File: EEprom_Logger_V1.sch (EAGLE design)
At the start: 25 parts, among them IC1 AP2138N-3.3TRG1, IC2 PIC18F13K22SOP, IC3 MIC94090, IC4 MCP1700T-2702E/TT, IC5 24LC16BSN, Q1 Si2333CDS-T1-GE3, Q2 Si2333CDS-T1-GE3, Y1 32kHz

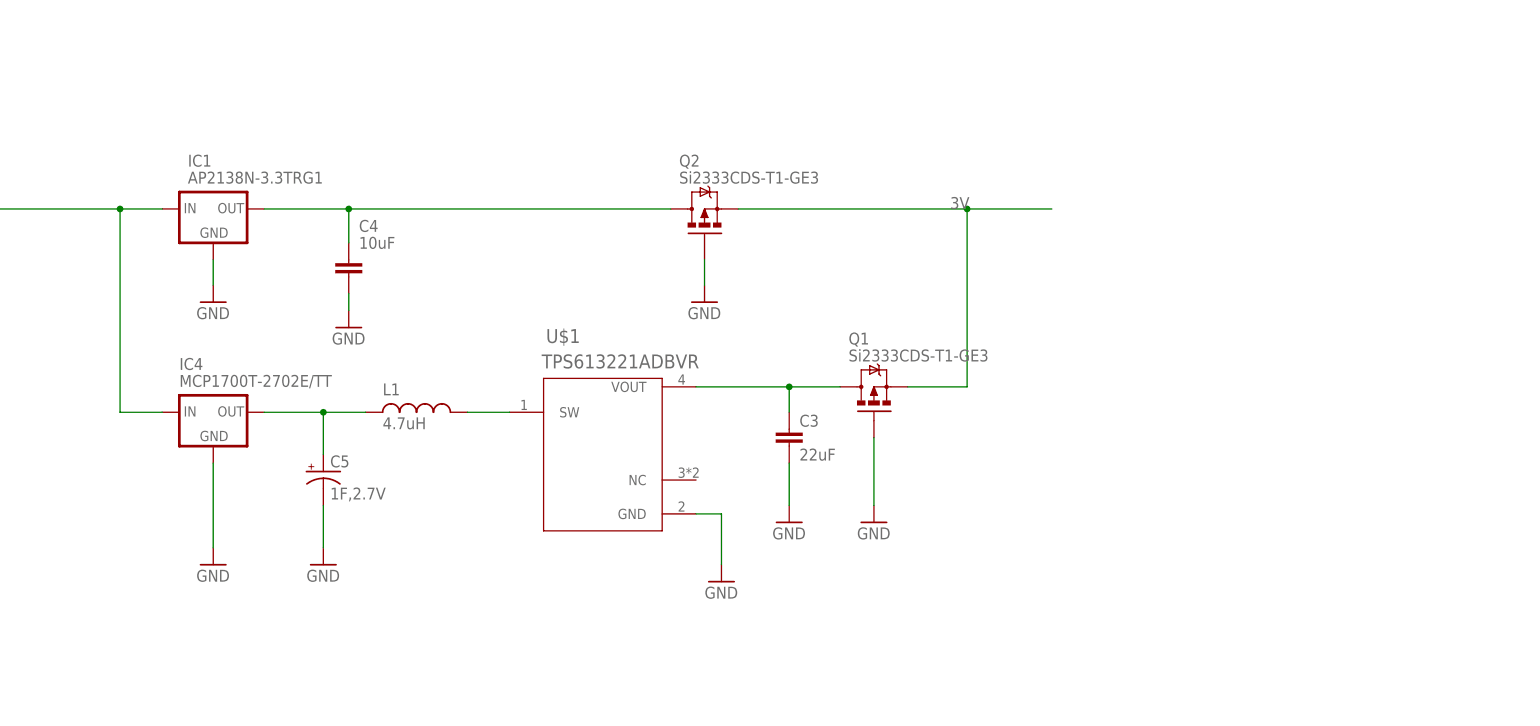
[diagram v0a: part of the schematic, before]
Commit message: Add files via upload
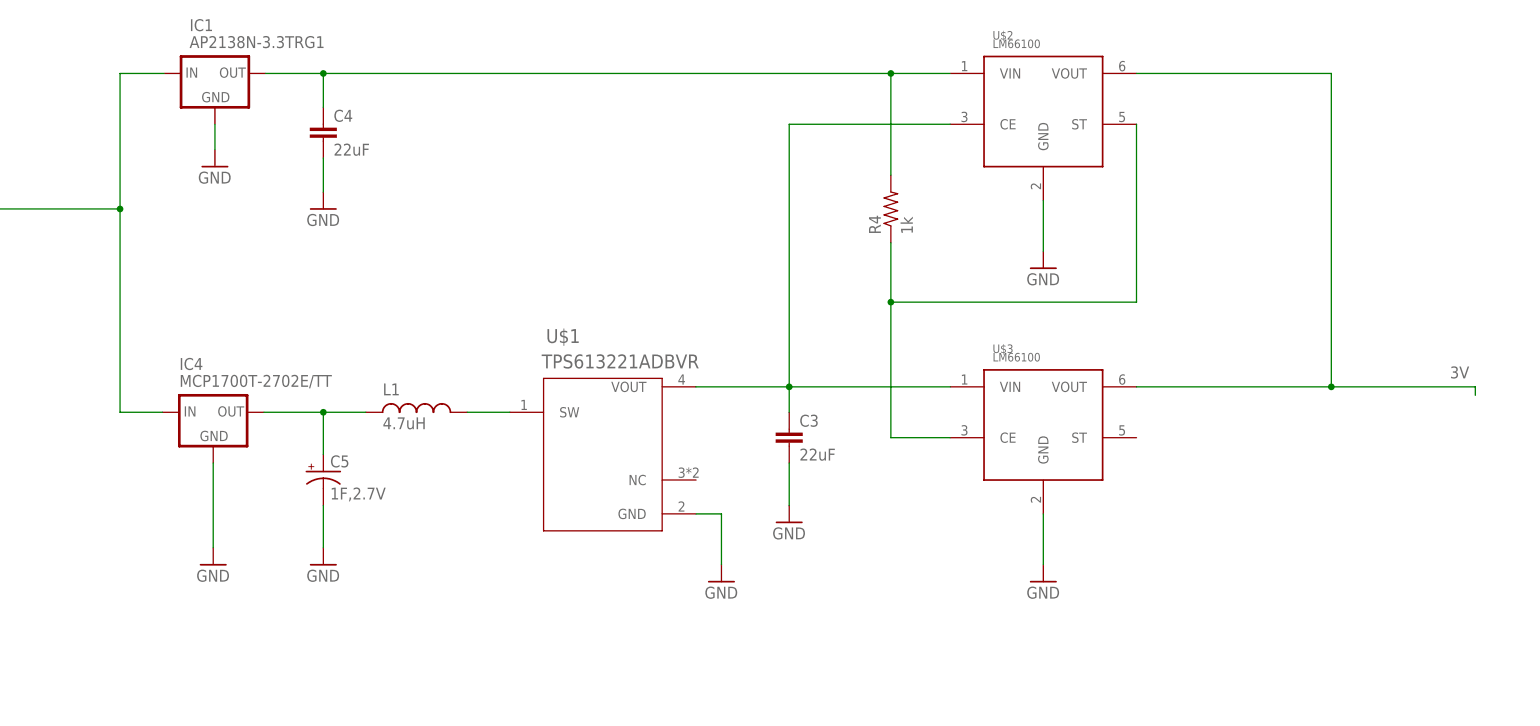
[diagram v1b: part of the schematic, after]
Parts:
- removed Q1, Q2: Si2333CDS-T1-GE3, SparkFun-DiscreteSemi:MOSFET-PCHANNEL
- added R4: 1k, SparkFun-Resistors:RESISTOR1206
- added U$2, U$3: LM66100, LM66100:LM66100
- C4: value 10uF -> 22uF
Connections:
- new net N$3: C4.2, IC1.OUT, R4.2, U$2.VIN
- net 3V: now also U$2.VOUT, U$3.VOUT; no longer Q1.S, Q2.S
- net GND: now also U$2.GND, U$3.GND; no longer Q1.G, Q2.G
- net N$6: now also R4.1, U$2.ST, U$3.CE; no longer C4.2, IC1.OUT, Q2.D
- net N$9: now also U$2.CE, U$3.VIN; no longer Q1.D
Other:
- moved on the sheet: C4, IC1
